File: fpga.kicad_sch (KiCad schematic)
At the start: 0 parts

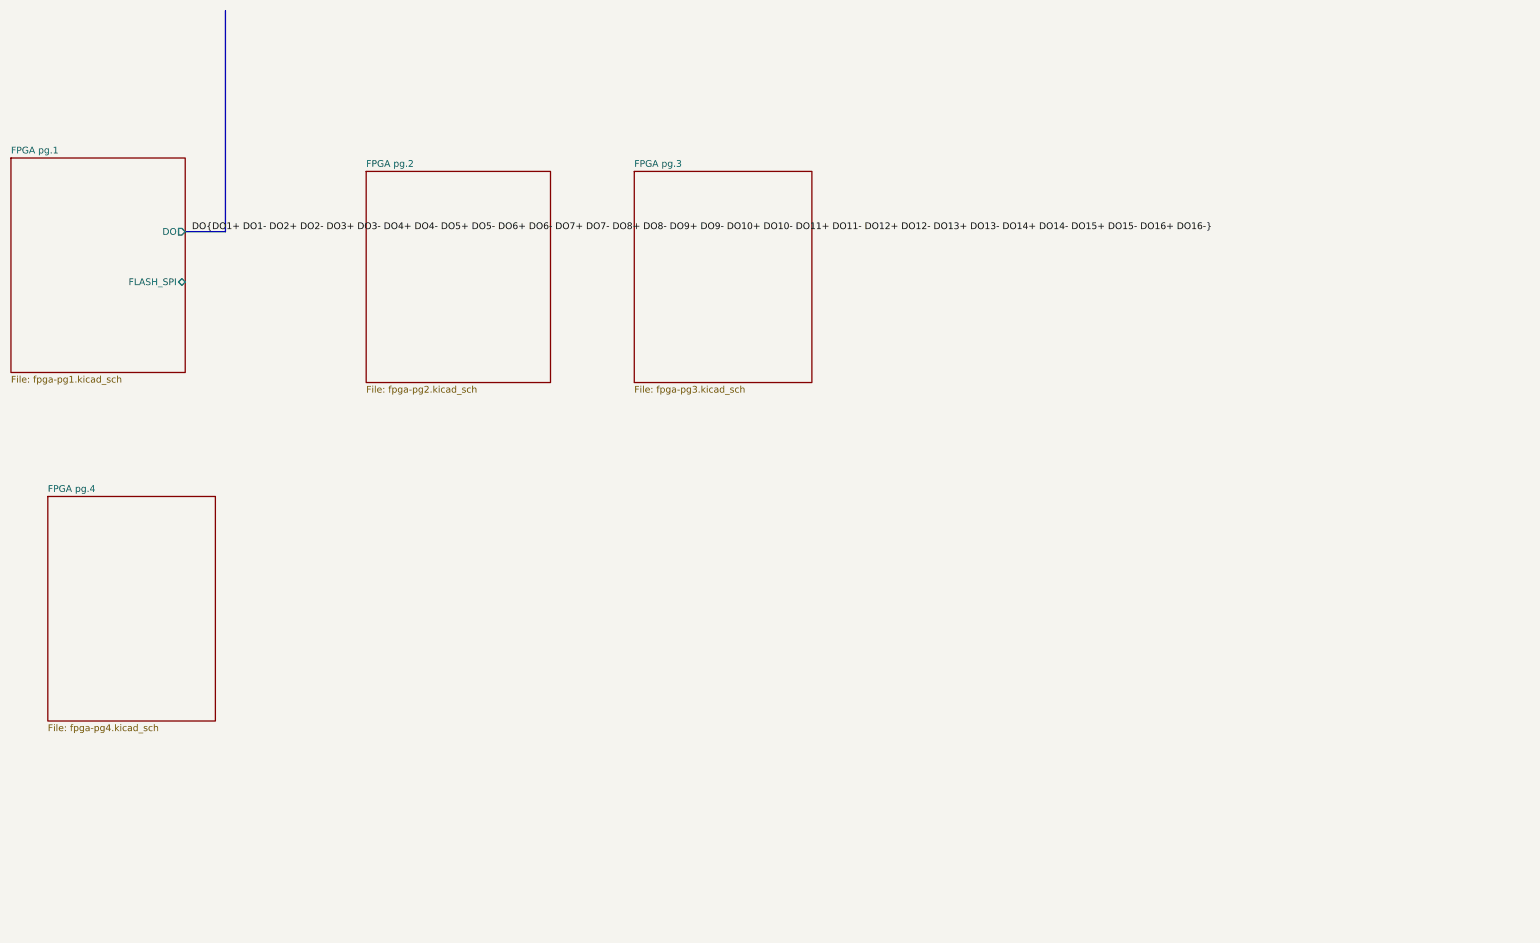
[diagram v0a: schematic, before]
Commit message: stuff
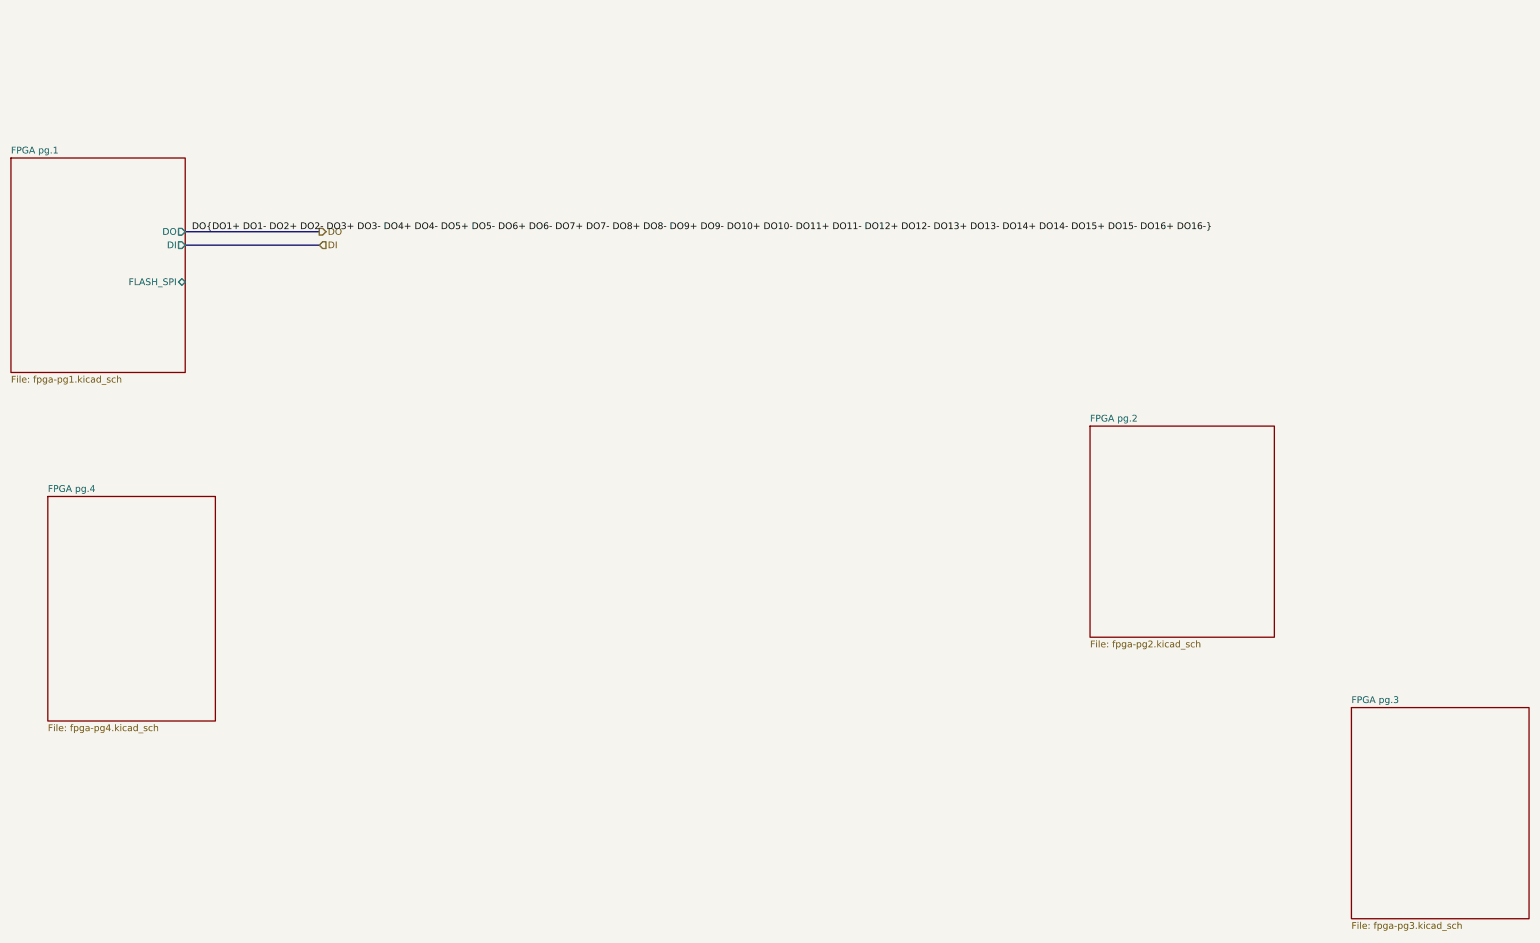
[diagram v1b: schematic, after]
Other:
- sheet FPGA pg.1 ports: added DI; removed none
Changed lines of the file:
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@@
 	(bus
 		(pts
-			(xy 99.06 34.29) (xy 99.06 76.2)
+			(xy 91.44 76.2) (xy 116.84 76.2)
 		)
 		(stroke
@@
 	(bus
 		(pts
-			(xy 91.44 76.2) (xy 99.06 76.2)
+			(xy 91.44 78.74) (xy 116.84 78.74)
 		)
 		(stroke
@@
 			)
 			(justify left bottom)
+		)
+	)
+	(hierarchical_label "DI"
+		(shape input)
+		(at 116.84 78.74 0)
+		(fields_autoplaced yes)
+		(effects
+			(font
+				(size 1.27 1.27)
+			)
+			(justify left)
+		)
+	)
+	(hierarchical_label "DO"
+		(shape output)
+		(at 116.84 76.2 0)
+		(fields_autoplaced yes)
+		(effects
+			(font
+				(size 1.27 1.27)
+			)
+			(justify left)
 		)
 	)
@@
 			)
 		)
+		(pin "DI" output
+			(at 91.44 78.74 0)
+			(effects
+				(font
+					(size 1.27 1.27)
+				)
+				(justify right)
+			)
+		)
 		(instances
 			(project "logix-core"
@@
 	)
 	(sheet
-		(at 176.53 64.77)
+		(at 312.42 166.37)
 		(size 33.655 40.005)
 		(fields_autoplaced yes)
@@
 		)
 		(property "Sheetname" "FPGA pg.3"
-			(at 176.53 64.0584 0)
+			(at 312.42 165.6584 0)
 			(effects
 				(font
@@
 		)
 		(property "Sheetfile" "fpga-pg3.kicad_sch"
-			(at 176.53 105.3596 0)
+			(at 312.42 206.9596 0)
 			(effects
 				(font
@@
 	)
 	(sheet
-		(at 125.73 64.77)
+		(at 262.89 113.03)
 		(size 34.925 40.005)
 		(fields_autoplaced yes)
@@
 		)
 		(property "Sheetname" "FPGA pg.2"
-			(at 125.73 64.0584 0)
+			(at 262.89 112.3184 0)
 			(effects
 				(font
@@
 		)
 		(property "Sheetfile" "fpga-pg2.kicad_sch"
-			(at 125.73 105.3596 0)
-			(effects
-				(font
+			(at 262.89 153.6196 0)
+			(effects
+				(font

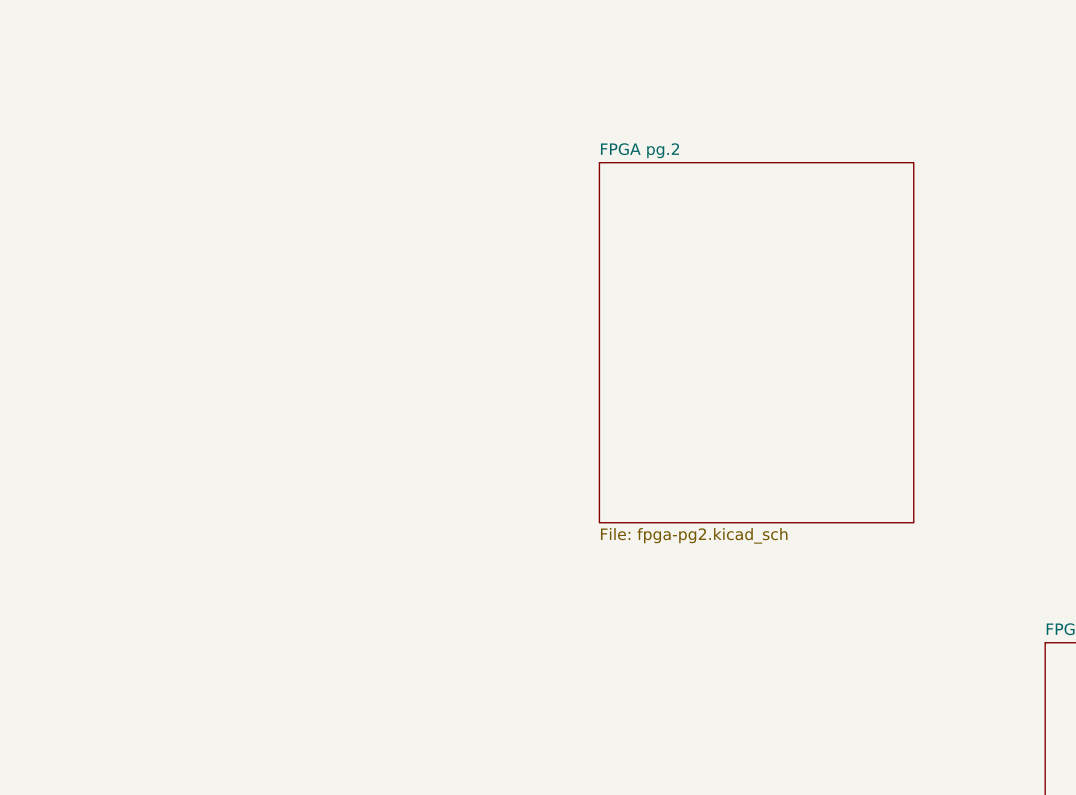
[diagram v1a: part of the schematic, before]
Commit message: working on ddr3
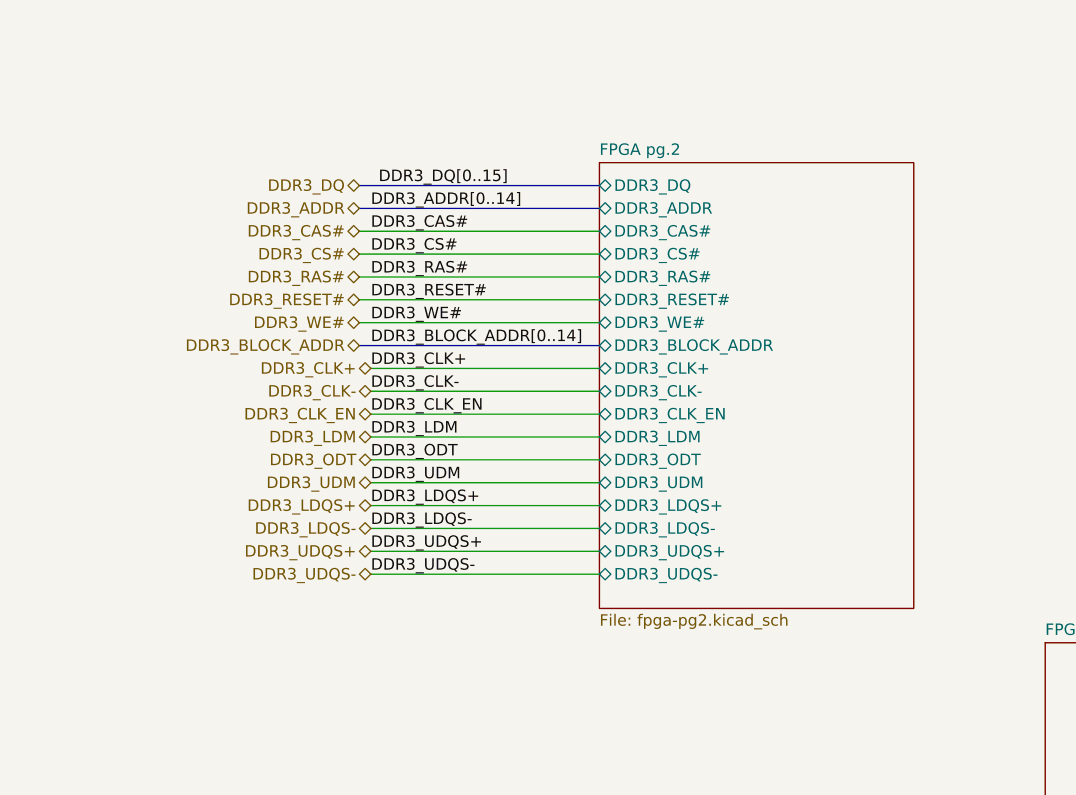
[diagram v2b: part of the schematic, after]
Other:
- sheet FPGA pg.2 ports: added DDR3_ADDR, DDR3_BLOCK_ADDR, DDR3_CAS#, DDR3_CLK+, DDR3_CLK-, DDR3_CLK_EN, DDR3_CS#, DDR3_DQ, DDR3_LDM, DDR3_LDQS+, DDR3_LDQS-, DDR3_ODT, DDR3_RAS#, DDR3_RESET#, DDR3_UDM, DDR3_UDQS+, DDR3_UDQS-, DDR3_WE#; removed none
